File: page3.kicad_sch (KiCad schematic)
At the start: 27 parts, among them U23 CD4094

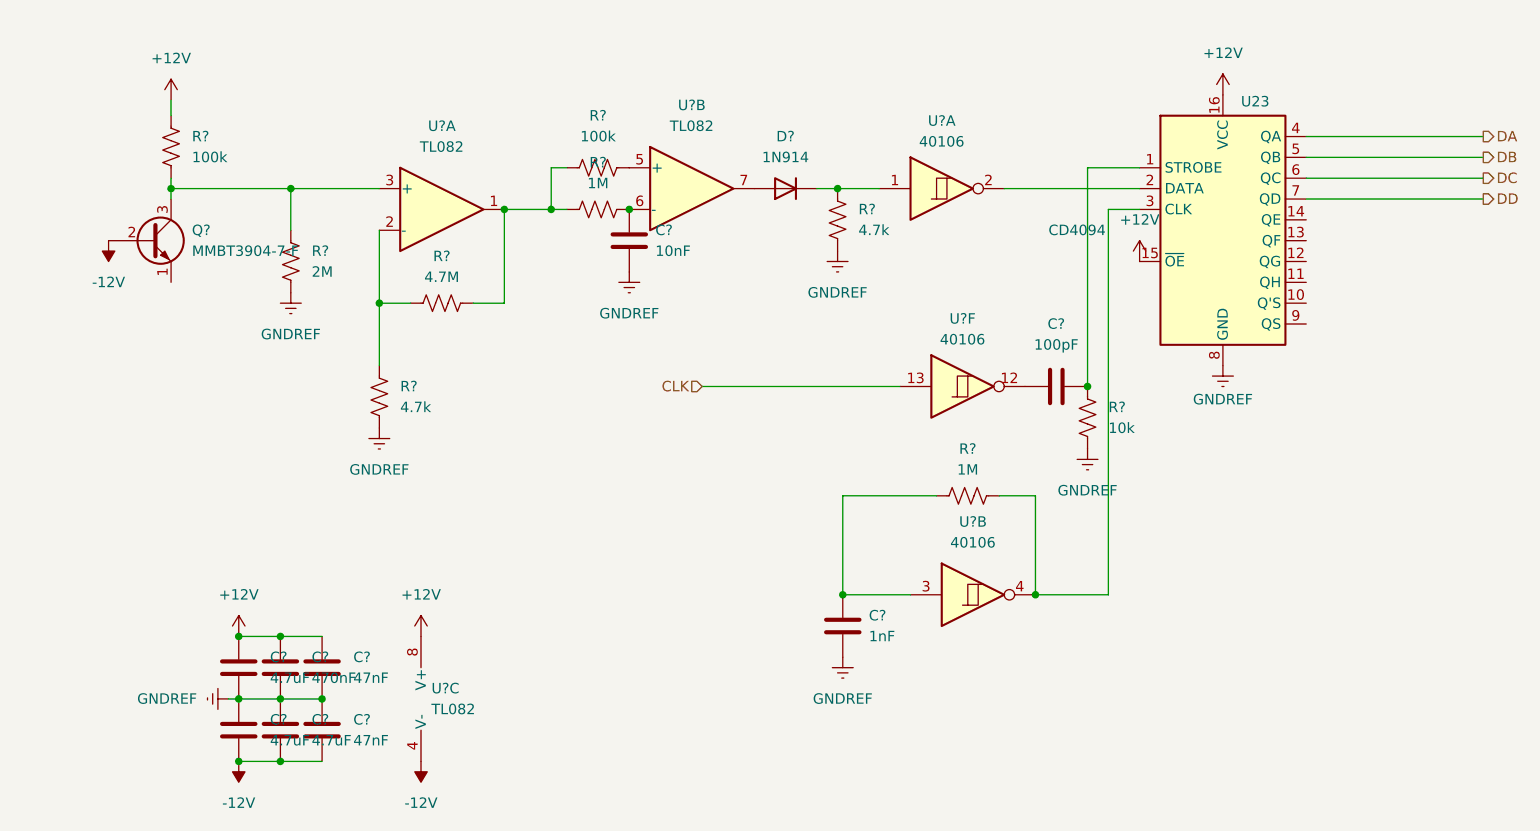
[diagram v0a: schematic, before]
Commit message: finishing schematic 1.0
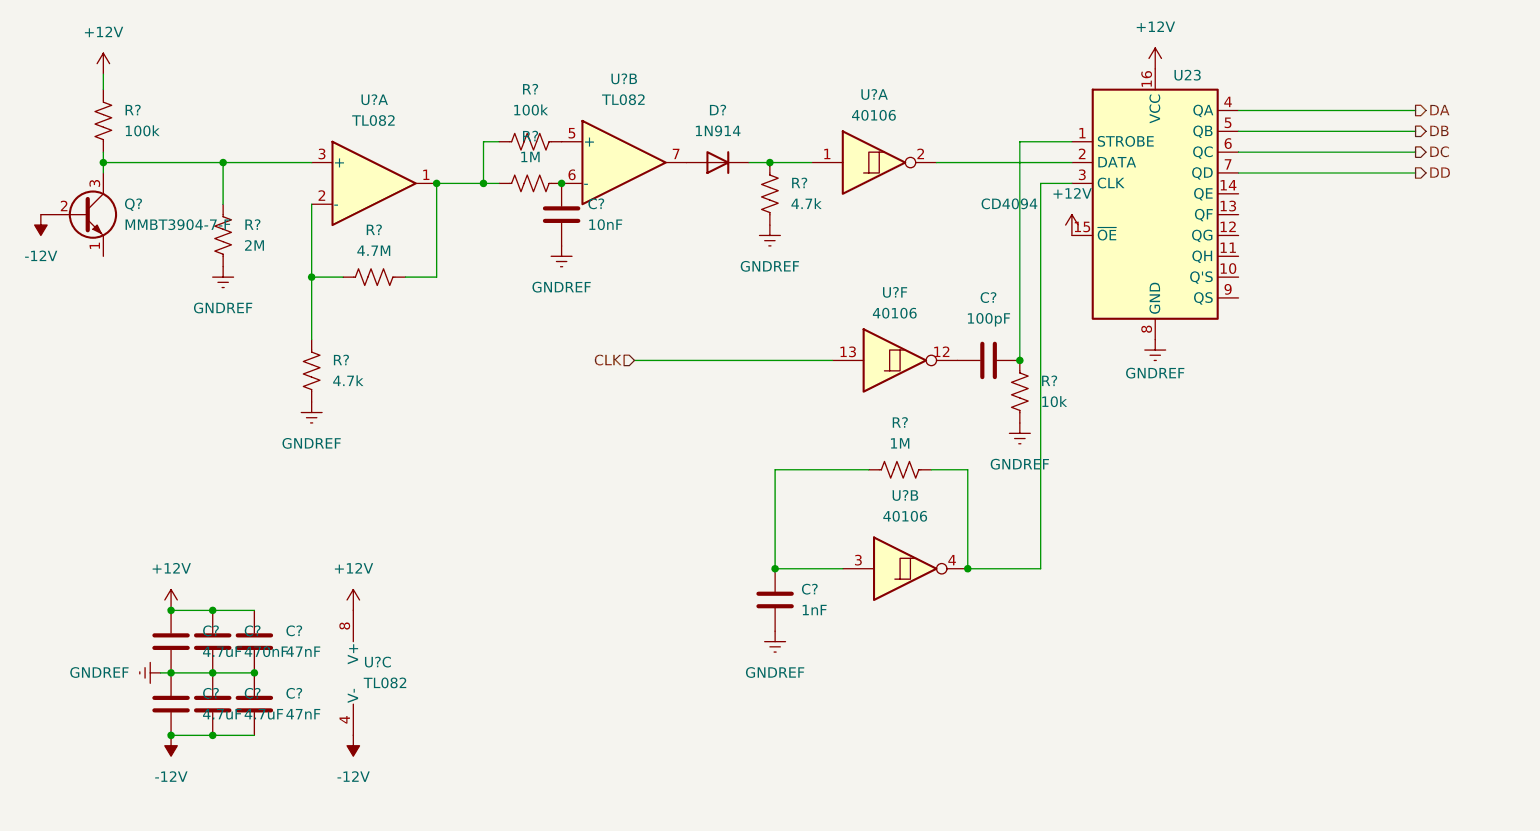
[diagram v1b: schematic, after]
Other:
- moved on the sheet: C?, D?, Q?, R?, U23, U?A, U?B, U?C, U?F
